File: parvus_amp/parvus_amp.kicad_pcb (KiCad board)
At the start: 2 copper layers, 86 x 60 mm, 40 parts, among them J1 input, J2 output, J3 powersupply, U1 LM3886

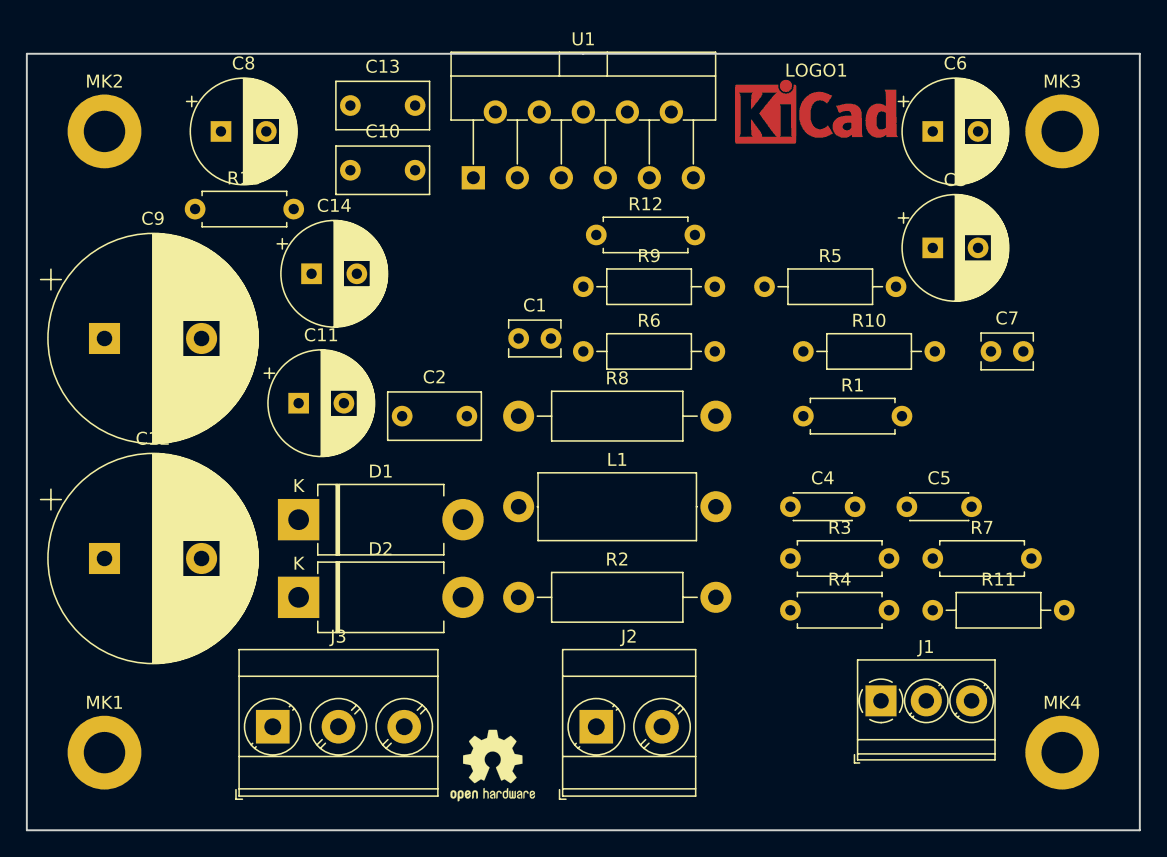
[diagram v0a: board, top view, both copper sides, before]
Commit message: Updated schematic and README description
Signed-off-by: Nenad Radulovic <nenad.b.radulovic@gmail.com>
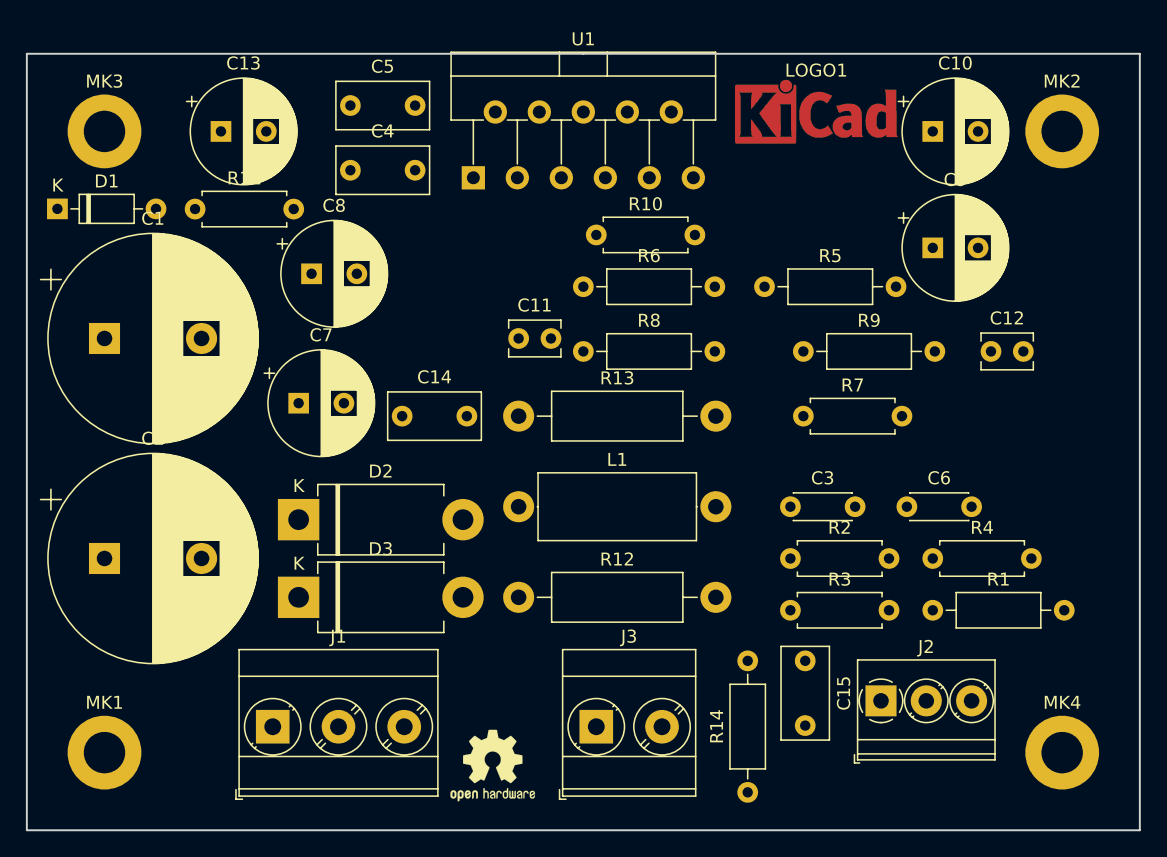
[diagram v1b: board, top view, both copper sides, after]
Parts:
- added C15: 100n, Capacitor_THT:C_Rect_L7.0mm_W3.5mm_P5.00mm, F.Cu at (152.6, 100.3)
- added D1: BZX85C16, Diode_THT:D_DO-35_SOD27_P7.62mm_Horizontal, F.Cu at (94.9, 65.4)
- added R14: 10, Resistor_THT:R_Axial_DIN0207_L6.3mm_D2.5mm_P10.16mm_Horizontal, F.Cu at (148.2, 110.5)
- R11: renamed from R13; value 100k -> 7k5
- renumbered C9 to C1, C6 to C10, C1 to C11, C7 to C12, C8 to C13, C2 to C14, C12 to C2, C4 to C3, C10 to C4, C13 to C5, C5 to C6, C11 to C7, C14 to C8, C3 to C9, D1 to D2, D2 to D3, J3 to J1, J1 to J2, J2 to J3, MK3 to MK2, MK2 to MK3, R11 to R1, R12 to R10, R2 to R12, R8 to R13, R3 to R2, R4 to R3, R7 to R4, R9 to R6, R1 to R7, R6 to R8, R10 to R9
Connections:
- C13 pad 2: Net-(C8-Pad2) -> Net-(C13-Pad2)
- R11 pad 1: Net-(C8-Pad2) -> Net-(C13-Pad2)
- U1 pad 8: Net-(C8-Pad2) -> Net-(D1-Pad1)
